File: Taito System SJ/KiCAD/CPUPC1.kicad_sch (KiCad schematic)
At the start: 44 parts, among them U11 74LS161, U13 74LS161, U17 74LS85, U18 74LS85, U19 74LS85, U21 74LS04, U24 74LS161, U26 74LS161, U34 74LS08, U36 74LS04, U37 74LS164, U38 74LS175, U51 74LS74, U61 74LS02, U62 74LS00, U63 74LS367, U74 74LS74, U75 74LS74, U88 74LS04, U94 74LS32, U97 74LS74

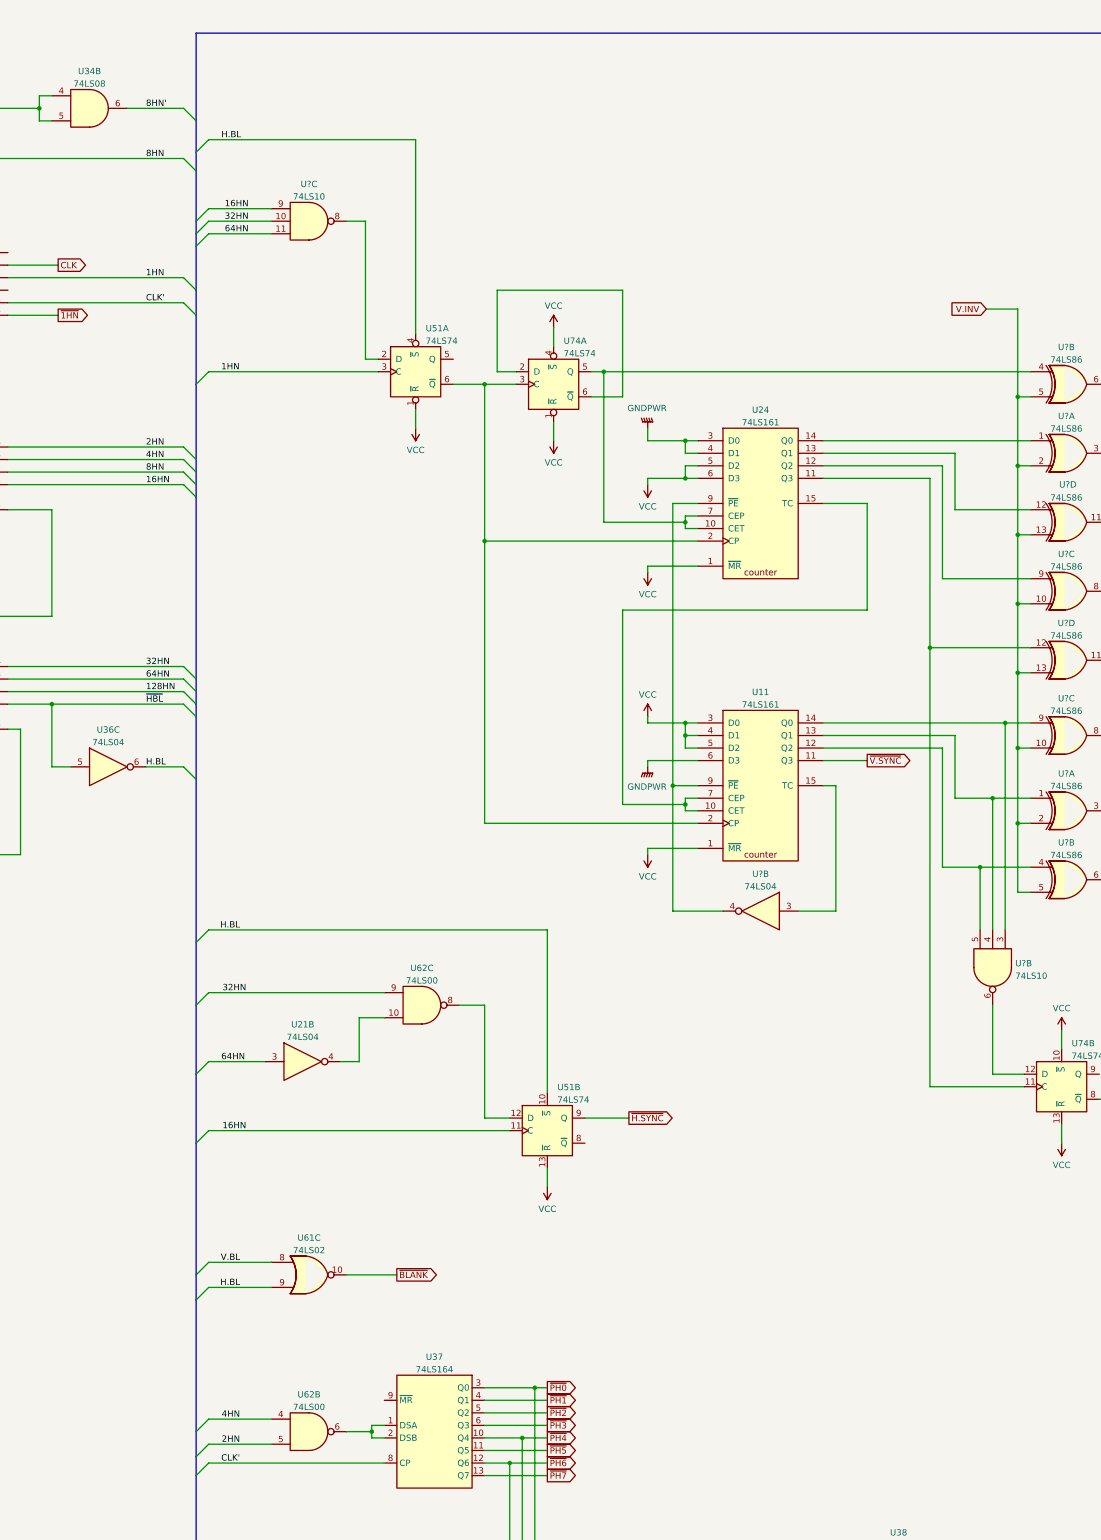
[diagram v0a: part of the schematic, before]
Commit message: Update before transfer
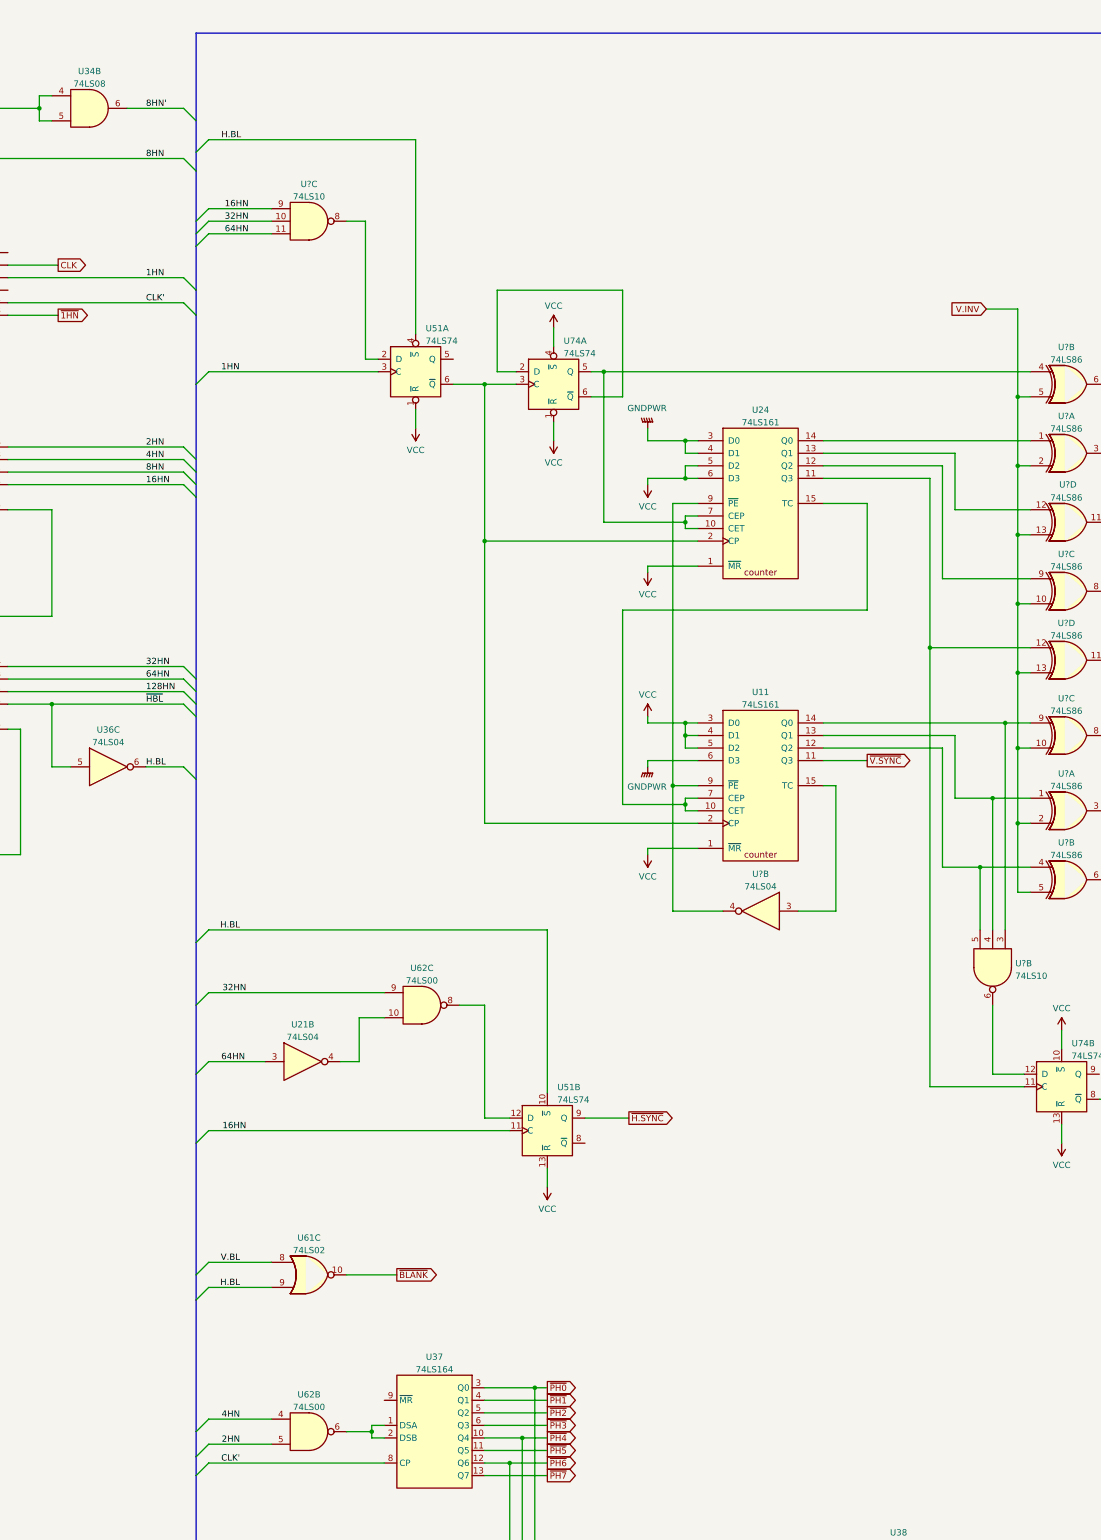
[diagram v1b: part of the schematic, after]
